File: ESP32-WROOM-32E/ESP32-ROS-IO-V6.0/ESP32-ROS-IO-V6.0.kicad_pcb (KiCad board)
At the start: 2 copper layers, 100 x 100 mm, 56 parts, among them J1 Conn_01x19_Socket, J16 XT60-M, J17 XT60-M, J2 Conn_01x19_Socket, J3 Conn_01x19_Socket, J4 Conn_01x19_Socket, SW1 SW1, SW2 SW2, SW3 SW3, SW4 SW4, SW5 SW5, SW6 SW6, SW7 SW7, SW8 SW7

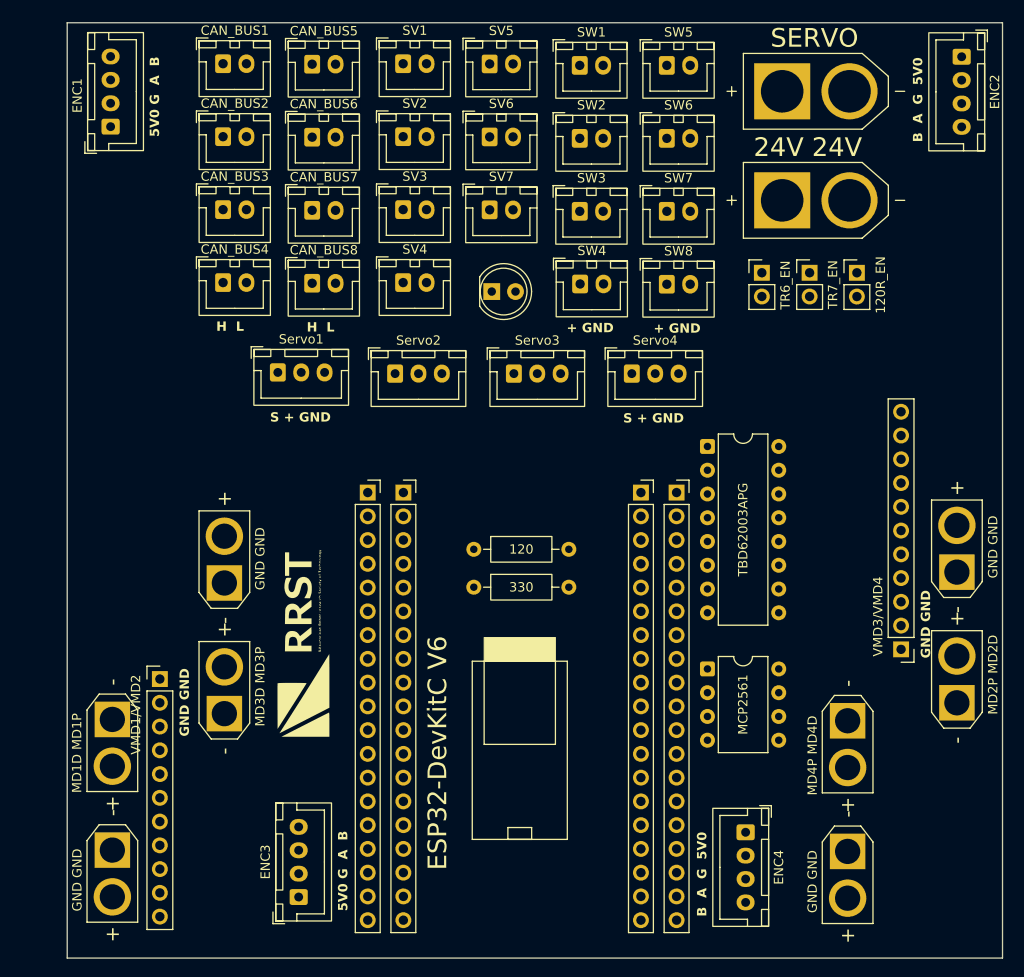
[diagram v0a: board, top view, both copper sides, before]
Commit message: 配線前
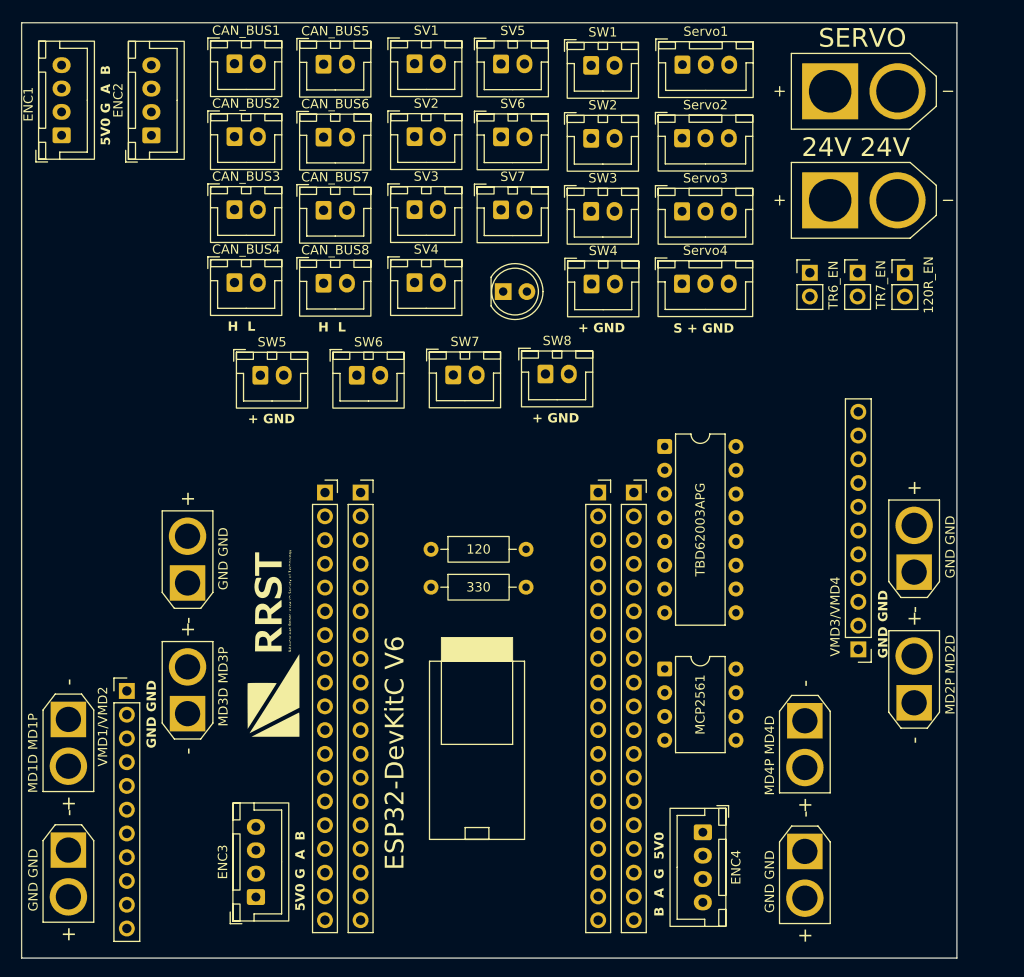
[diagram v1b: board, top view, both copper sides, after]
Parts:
- moved ENC2 87.0 mm to (108.9, 63.8), turned to 90 degrees
- moved SW5 54.6 mm to (120.6, 89.4)
- moved Servo1 54.4 mm to (165.7, 56.2)
- moved SW6 41.7 mm to (130.9, 89.4)
- moved Servo2 39.7 mm to (165.7, 64.1)
- moved SW7 28.8 mm to (141.2, 89.4)
- moved Servo3 25.0 mm to (165.7, 71.9)
- moved SW8 16.1 mm to (151.1, 89.3)
- moved Servo4 11.0 mm to (165.7, 79.7)
- moved ENC1 5.32 mm to (99.3, 63.8)
- moved J16 5.13 mm to (185.1, 59.1)
- moved J17 5.13 mm to (185.1, 70.7)
- moved 120R_EN 5.13 mm to (189.5, 78.5)
- moved TR6_EN 5.13 mm to (179.3, 78.5)
- moved TR7_EN 5.13 mm to (184.5, 78.5)
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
